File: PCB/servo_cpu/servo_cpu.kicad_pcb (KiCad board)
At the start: 4 copper layers, 96 x 172 mm, 166 parts, among them J1 PWR board, J2 Control power, J3 ABZ, J4 Serial Encoder, J5 CONN, J6 DEBUG, J7 USB_B, J8 I/O, J9 EXT, SW1 ENTER, SW2 ESC, SW3 UP, SW4 DOWN, U1 STM32F407VETx, U10 SN65HVD232, U11 LMC7660, U12 TS912, U13 74HC14, U14 ISP742RI, U15 ISP742RI, U16 TS912, U17 VO0661T, U18 74LVC2G04, U2 M24C02-WMN, U3 TS912, U4 AP1117-33, U5 ISL83491, U6 AP63205WU, U7 AM26LS32A, U8 AP2151A, U9 MAX485E, Y1 16M xt224

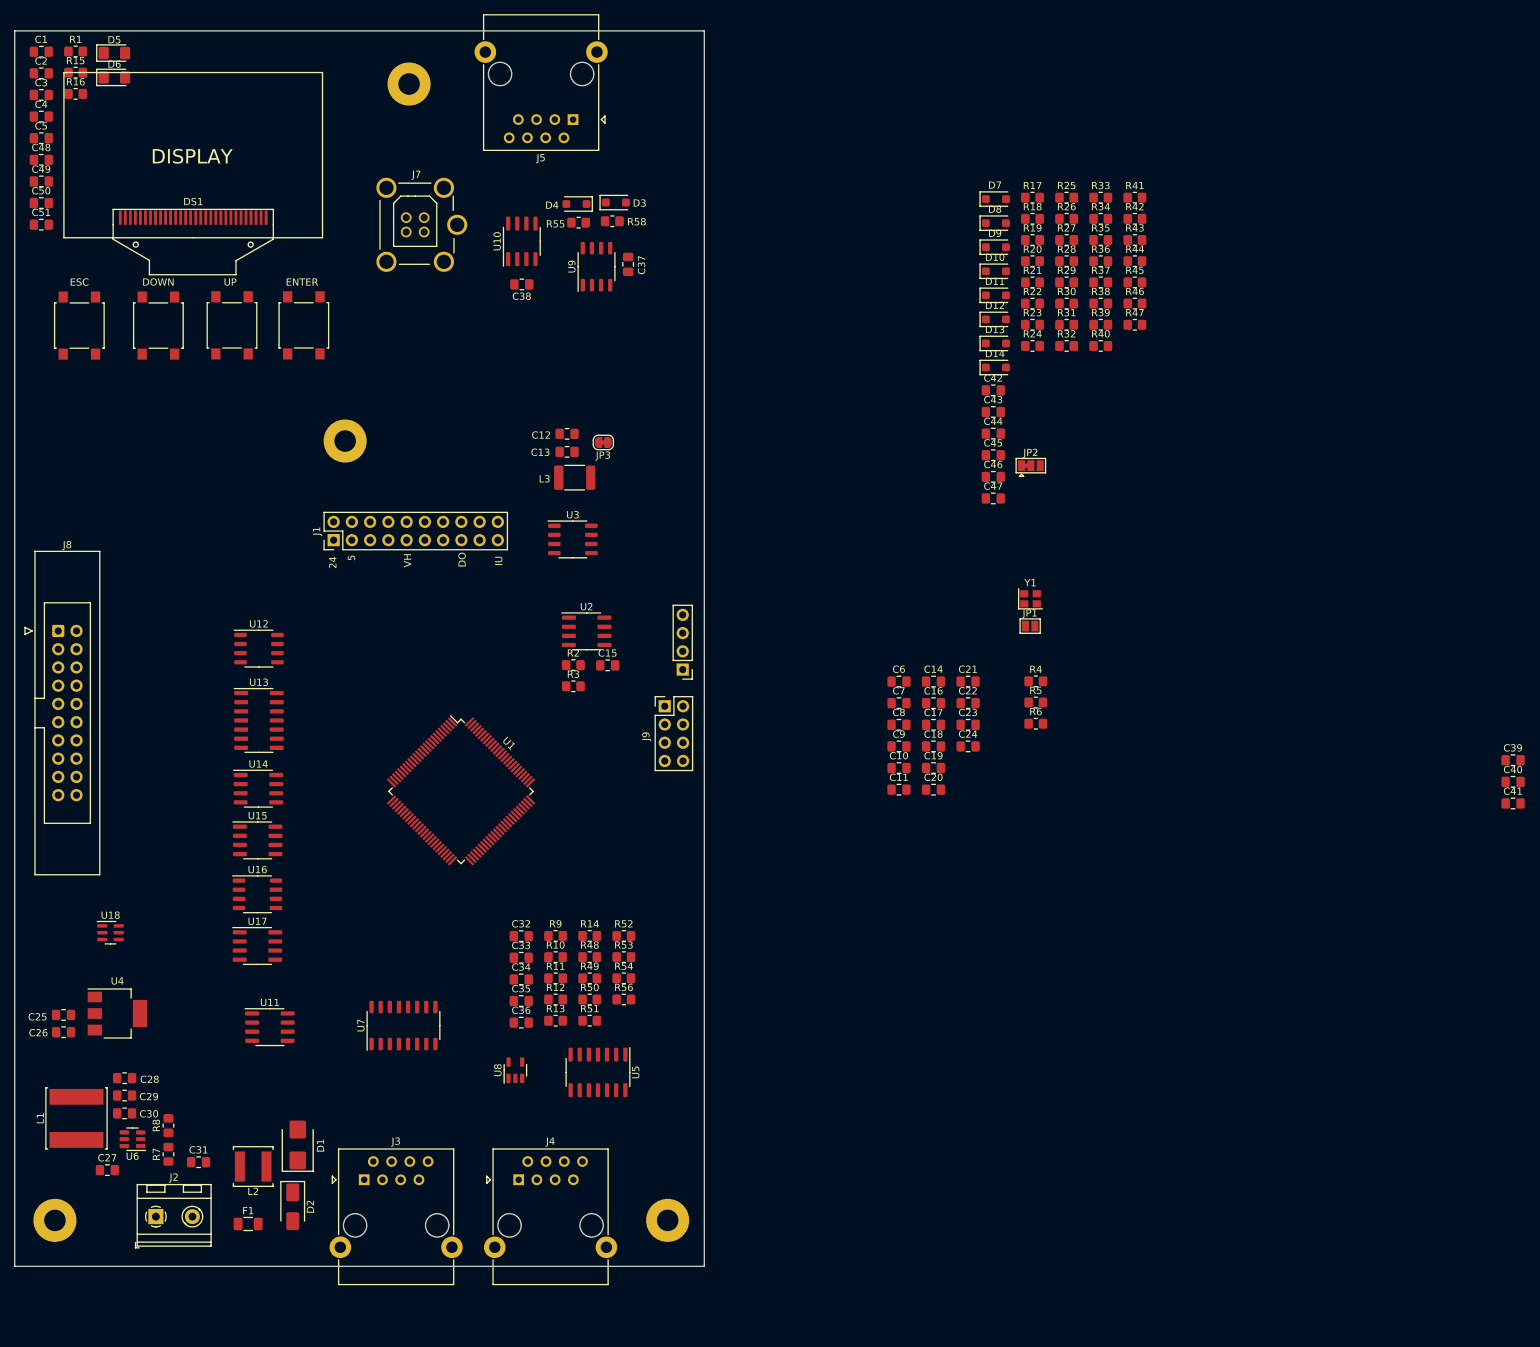
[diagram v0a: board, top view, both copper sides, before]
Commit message: cpu pcb routing
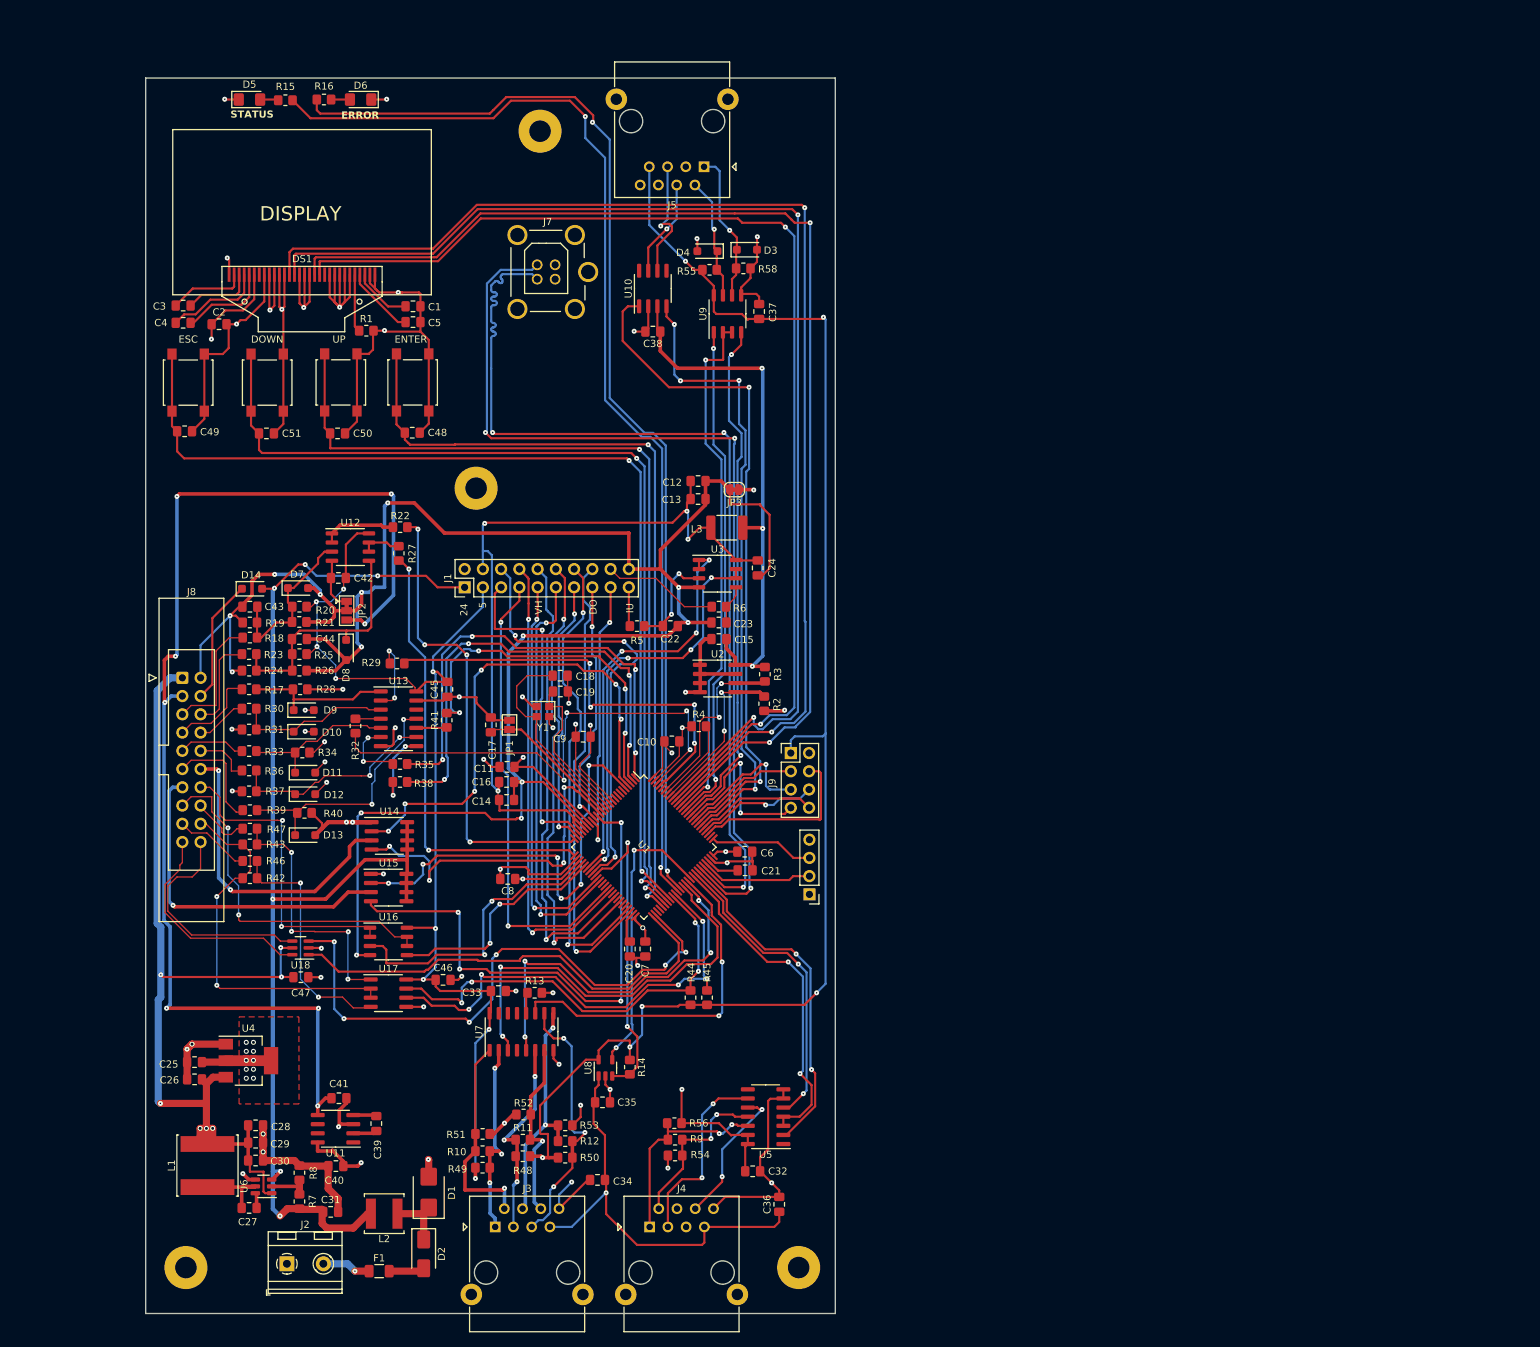
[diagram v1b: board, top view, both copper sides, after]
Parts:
- moved C40 172.4 mm to (95.5, 170.4), turned to 180 degrees
- moved C41 168.5 mm to (95.9, 161.0)
- moved C39 166.1 mm to (101.1, 164.5), turned to 90 degrees
- moved R42 153.6 mm to (83.5, 130.4), turned to 180 degrees
- moved R43 149.2 mm to (83.5, 125.7)
- moved R46 145.6 mm to (83.5, 128.0)
- moved R47 141.8 mm to (83.5, 123.5)
- moved R33 141.4 mm to (83.4, 112.7), turned to 180 degrees
- moved R36 138.1 mm to (83.4, 115.4), turned to 180 degrees
- moved R37 138.1 mm to (83.4, 118.3)
- moved R39 136.4 mm to (83.5, 120.9), turned to 180 degrees
- moved R34 133.7 mm to (90.8, 112.9), turned to 180 degrees
- moved R17 128.8 mm to (83.4, 104.1), turned to 180 degrees
- moved R40 128.5 mm to (91.1, 121.3), turned to 180 degrees
- moved R30 127.0 mm to (83.4, 106.8), turned to 180 degrees
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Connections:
- C14 pad 2: GND -> GNDA
- U1 pad 96: MODBUS_DE -> unconnected-(U1-PB9-Pad96)
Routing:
- net +5V: track 0.00 -> 498.3 mm, vias 0 -> 23
- net GND: track 0.00 -> 416.7 mm, vias 0 -> 56
- net GNDA: track 0.00 -> 303.0 mm, vias 0 -> 14
- net +3V3: track 0.00 -> 185.4 mm, vias 0 -> 23
- net /DISPLAY_CS: track 0.00 -> 171.0 mm, vias 0 -> 2
- net +24V: track 0.00 -> 169.8 mm, vias 0 -> 6
- net /DISPLAY_RESET: track 0.00 -> 169.3 mm, vias 0 -> 2
- net -5V: track 0.00 -> 167.0 mm, vias 0 -> 8
- net DISPLAY_CLK: track 0.00 -> 166.0 mm, vias 0 -> 2
- net DISPLAY_MOSI: track 0.00 -> 159.0 mm, vias 0 -> 2
- net LED_STATUS: track 0.00 -> 157.8 mm, vias 0 -> 2
- net LED_ERROR: track 0.00 -> 155.6 mm, vias 0 -> 2
- net BTN_ESC: track 0.00 -> 140.7 mm, vias 0 -> 2
- net USB_N: track 0.00 -> 136.4 mm, vias 0 -> 3
- net USB_P: track 0.00 -> 136.2 mm, vias 0 -> 3
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- added copper zone on F.Cu, net +3V3
- added copper zone on In1.Cu, net +3V3
- added copper zone on In1.Cu, net +5V
- added copper zone on In2.Cu, net GND
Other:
- board text added: "ERROR"
- board text added: "STATUS"
